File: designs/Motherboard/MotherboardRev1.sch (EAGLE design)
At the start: 101 parts, among them IC3 PIC18F26J53ML, J1 Servo 2, J10 22-05-7028-02, J11 22-05-7028-02, J12 22-05-7028-02, J13 22-05-7048-04, J2 Servo 1, J3 Servo 3, J4 Servo 4, J5 Servo 5, J6 Servo 6, J7 22-05-7028-02, J8 22-05-7028-02, J9 22-05-7028-02, Q1 BSS123, Q2 BSS123, Q3 BSS123, Q4 BSS123, U1 TPS5450DDAR, U2 TPS5450DDAR, U3 LMS8117AMP-3.3

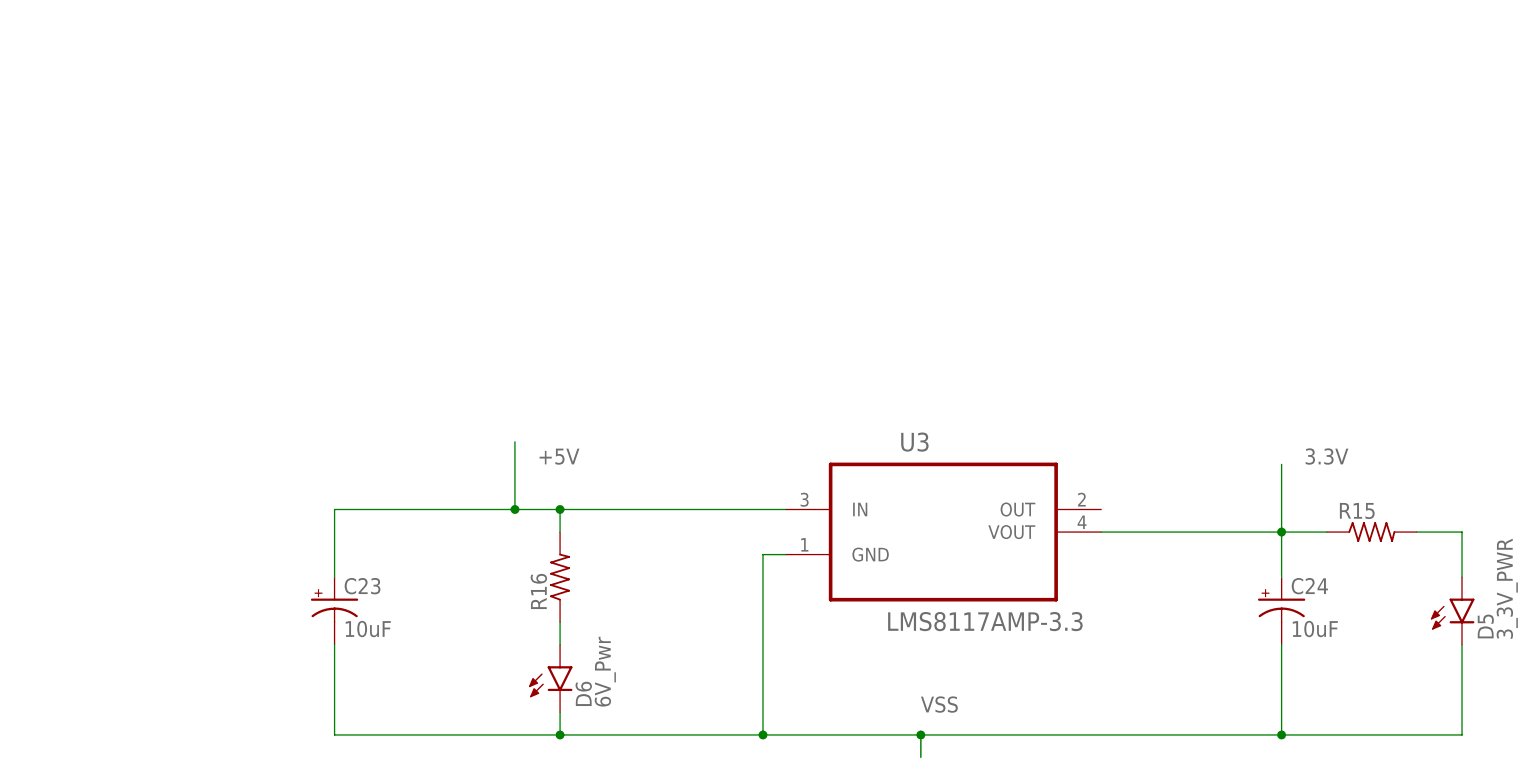
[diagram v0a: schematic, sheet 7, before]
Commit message: last commit of rev 1
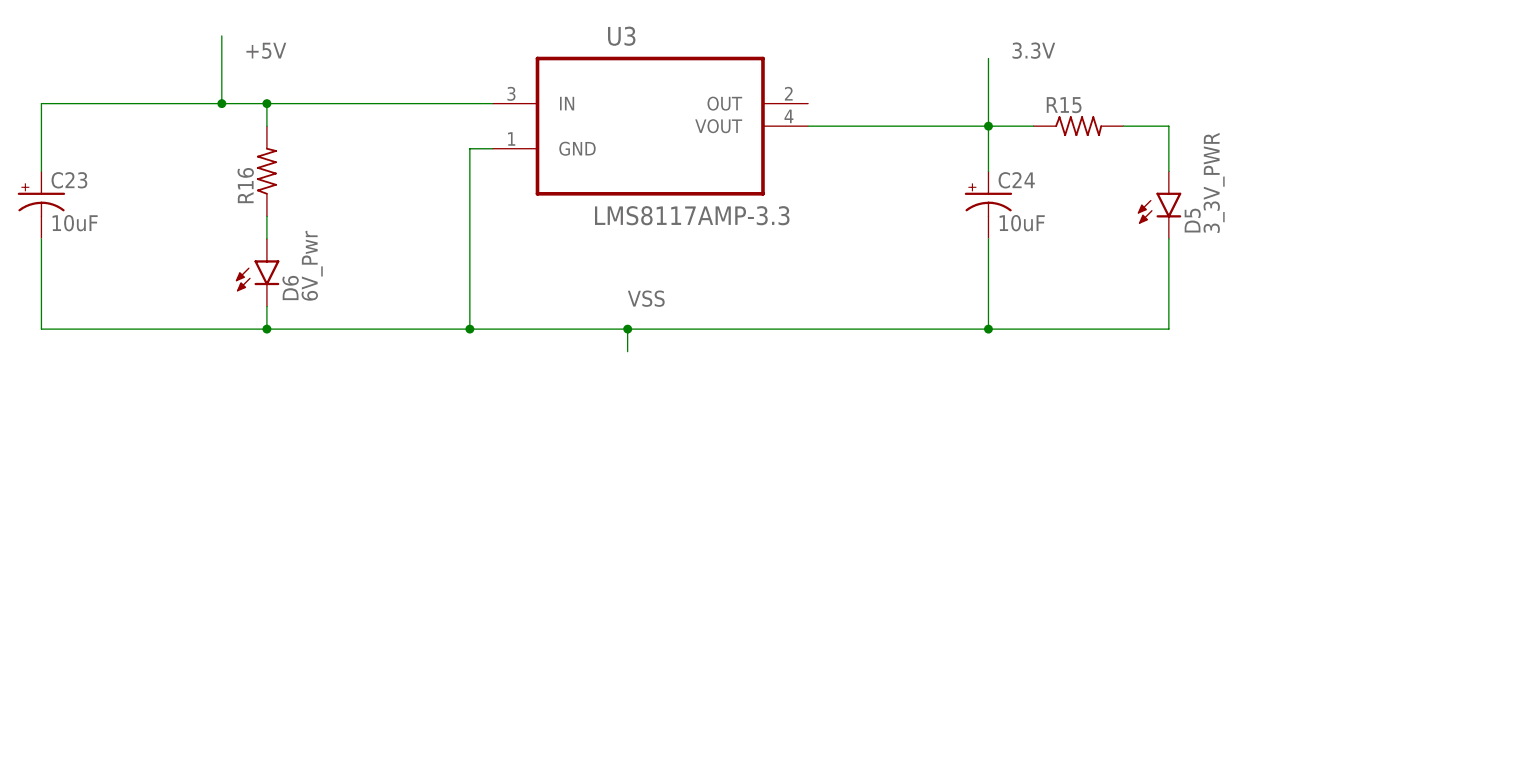
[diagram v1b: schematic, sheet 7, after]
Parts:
- added IC1: PIC18F26J53ML, microchip:PIC18F26J53ML
- added IC2: (no value), ic-package:DIL16
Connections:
- new net 1,2EN: IC2.1
- new net 1A: IC2.2
- new net 1Y: IC2.3
- new net 2A: IC2.7
- new net 2Y: IC2.6
- new net 3,4EN: IC2.9
- new net 3A: IC2.10
- new net 3Y: IC2.11
- new net 4A: IC2.15
- new net 4Y: IC2.14
- new net IO3(1): IC1.OSC2/CLKO/RA6
- new net IO5(1): IC1.VUSB
- new net IO7(1): IC1.RC5/D+/VP
- new net IO8(1): IC1.RA1/AN1/C2INA/VBG/RP1
- new net MCLR'(1): IC1.!MCLR
- new net N$19: IC2.8
- new net N$20: IC2.16
- new net OC4(1): IC1.RB1/AN10/C3INC/RTCC/RP4
- new net OC5(1): IC1.RB0/AN12/C3IND/INT0/RP3
- new net OC6(1): IC1.RC7/CCP10/RX1/DT1/SDO1/RP18
- new net PGC1(1): IC1.RA3/AN3/C1INB/VREF+
- new net PGD1(1): IC1.RA2/AN2/C2INB/C1IND/C3INB/VREF-/CVREF
- net 3.3V: now also IC1.RB7/CCP7/KBI3/PGD/RP10, IC1.RC2/AN11/C2IND/CTPLS/RP13
- net GND: now also IC1.RB6/CCP6/KBI2/PGC/RP9, IC1.VSS1, IC2.12, IC2.13, IC2.4, IC2.5
- net IO4: now also IC1.RC1/CCP8/T1OSI/!UOE!/RP12
- net IO6: now also IC1.RC4/D-/VM
- net N$25: now also IC1.RC0/T1OSO/T1CKI/RP11
- net N$31: now also IC1.RC6/CCP9/TX1/CK1/RP17
- net OC1: now also IC1.RB5/CCP5/KBI1/SDI1/SDA1/RP8
- net OC2: now also IC1.RB4/CCP4/KBI0/SCK1/SCL1/RP7
- net OC3: now also IC1.RB3/AN9/C3INA/CTED2/VPO/RP6
- net SCL: now also IC1.RA5/AN4/C1INC/!SS1!/HLVDIN/RCV/RP2
- net SDA: now also IC1.VDDCORE/VCAP
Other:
- moved on the sheet: C23, C24, D5, D6, R15, R16, U3
